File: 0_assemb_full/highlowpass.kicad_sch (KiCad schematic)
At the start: 21 parts, among them U3 LM2902, U4 LM2902

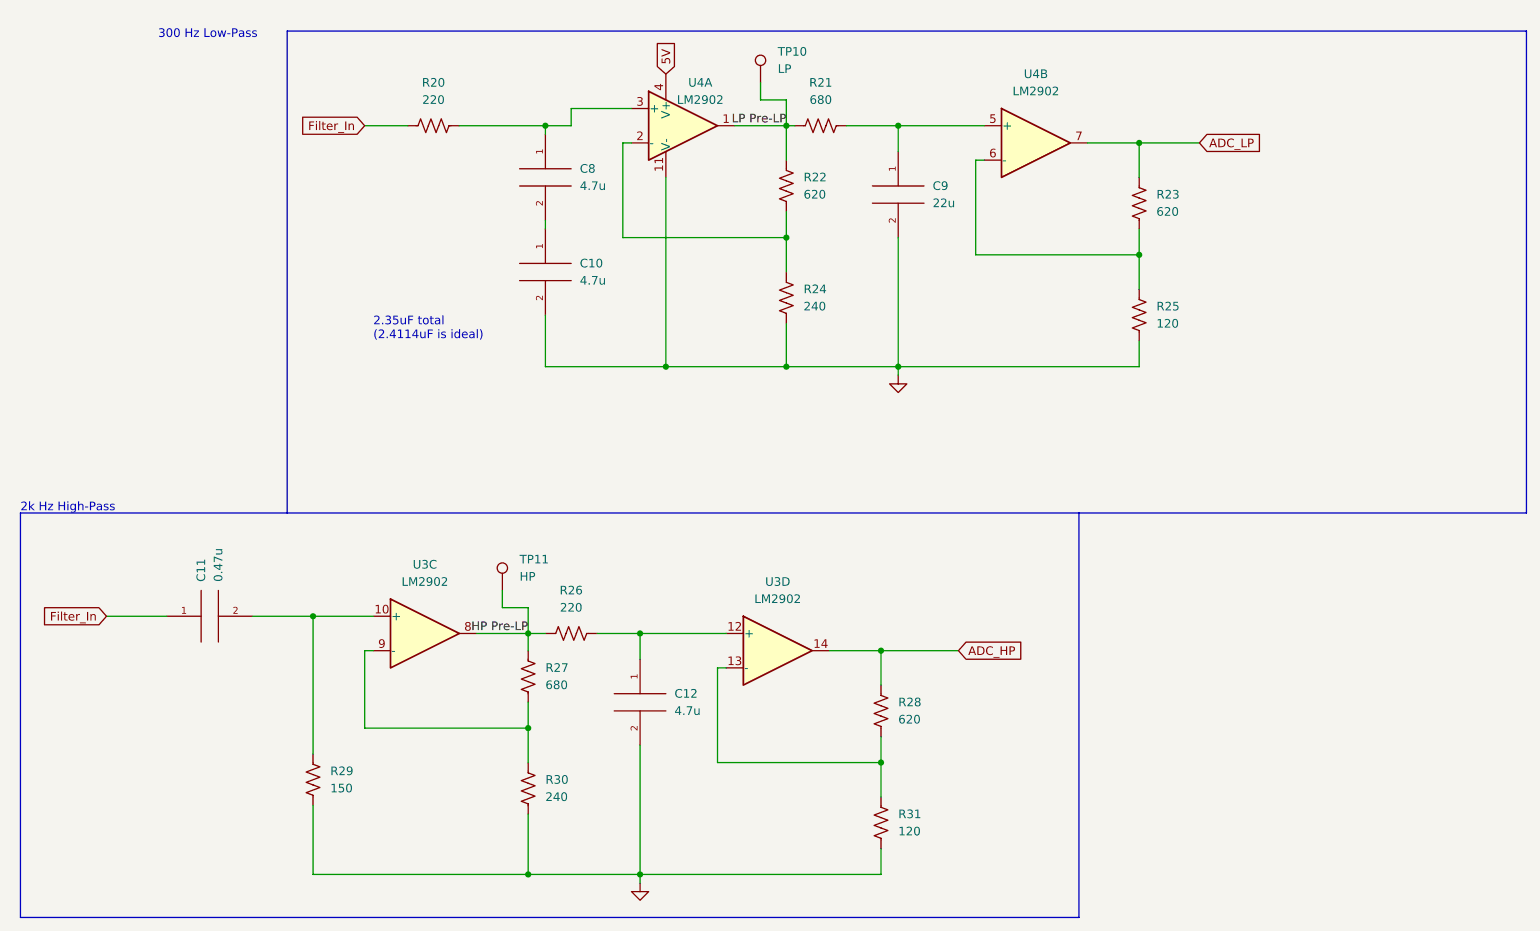
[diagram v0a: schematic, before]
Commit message: Some filter adjustments
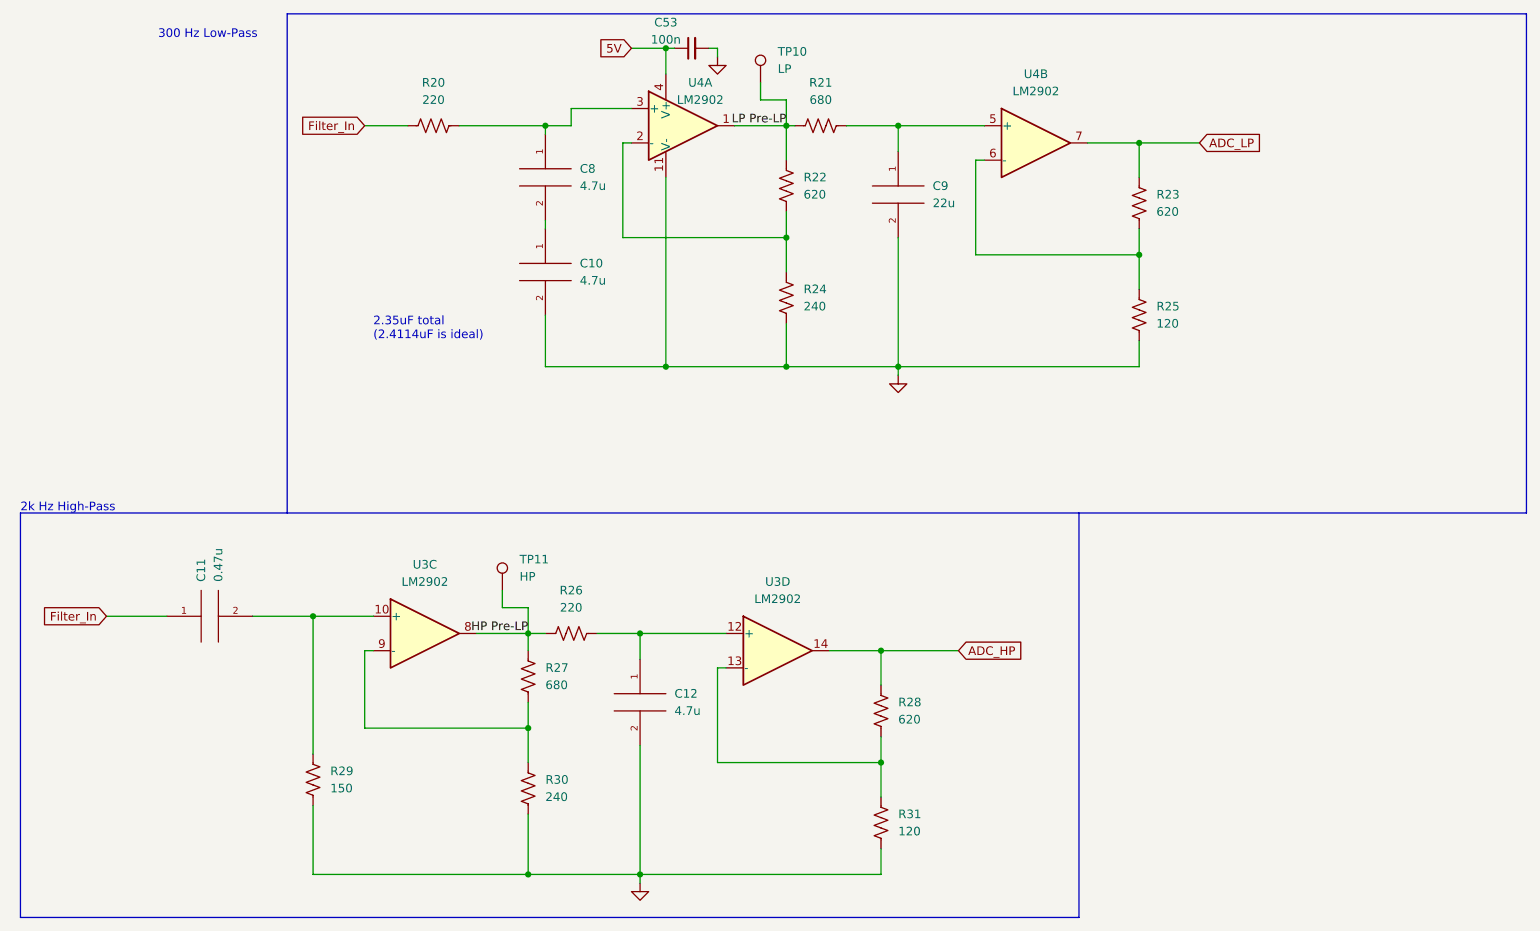
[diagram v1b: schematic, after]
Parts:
- added C53: 100n, Capacitor_SMD:C_0805_2012Metric_Pad1.18x1.45mm_HandSolder, symbol Device:C_Small
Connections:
- net 5V: now also C53.1
- net GND: now also C53.2
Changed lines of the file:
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@@
   (junction (at 179.07 31.75) (diameter 0) (color 0 0 0 0)
   )
+  (junction (at 109.22 17.78) (diameter 0) (color 0 0 0 0)
+  )
   (wire (pts (xy 143.51 45.72) (xy 143.51 64.77))
     (stroke (width 0) (type default) (color 0 0 0 0))
@@
     (stroke (width 0) (type default) (color 0 0 0 0))
   )
-  (polyline (pts (xy 236.22 86.36) (xy 236.22 15.24))
+  (polyline (pts (xy 236.22 86.36) (xy 236.22 12.7))
     (stroke (width 0) (type default) (color 0 0 0 0))
   )
@@
     (stroke (width 0) (type default) (color 0 0 0 0))
   )
-  (polyline (pts (xy 236.22 15.24) (xy 53.34 15.24))
+  (polyline (pts (xy 236.22 12.7) (xy 53.34 12.7))
     (stroke (width 0) (type default) (color 0 0 0 0))
   )
@@
     (stroke (width 0) (type default) (color 0 0 0 0))
   )
+  (wire (pts (xy 109.22 17.78) (xy 110.49 17.78))
+    (stroke (width 0) (type default) (color 0 0 0 0))
+  )
   (wire (pts (xy 127 29.21) (xy 127 34.29))
     (stroke (width 0) (type default) (color 0 0 0 0))
@@
     (stroke (width 0) (type default) (color 0 0 0 0))
   )
+  (wire (pts (xy 116.84 19.05) (xy 116.84 17.78))
+    (stroke (width 0) (type default) (color 0 0 0 0))
+  )
   (wire (pts (xy 88.9 100.33) (xy 88.9 104.14))
     (stroke (width 0) (type default) (color 0 0 0 0))
   )
-  (polyline (pts (xy 53.34 15.24) (xy 53.34 86.36))
+  (polyline (pts (xy 53.34 12.7) (xy 53.34 86.36))
     (stroke (width 0) (type default) (color 0 0 0 0))
   )
@@
     (stroke (width 0) (type default) (color 0 0 0 0))
   )
+  (wire (pts (xy 104.14 17.78) (xy 109.22 17.78))
+    (stroke (width 0) (type default) (color 0 0 0 0))
+  )
   (wire (pts (xy 104.14 31.75) (xy 102.87 31.75))
     (stroke (width 0) (type default) (color 0 0 0 0))
   )
+  (wire (pts (xy 116.84 17.78) (xy 115.57 17.78))
+    (stroke (width 0) (type default) (color 0 0 0 0))
+  )
   (wire (pts (xy 88.9 114.3) (xy 88.9 118.11))
     (stroke (width 0) (type default) (color 0 0 0 0))
@@
   )
   (wire (pts (xy 88.9 118.11) (xy 88.9 123.19))
+    (stroke (width 0) (type default) (color 0 0 0 0))
+  )
+  (wire (pts (xy 109.22 17.78) (xy 109.22 21.59))
     (stroke (width 0) (type default) (color 0 0 0 0))
   )
@@
     (effects (font (size 1.27 1.27)) (justify right bottom))
   )
-  (global_label "5V" (shape input) (at 109.22 21.59 90) (fields_autoplaced)
-    (effects (font (size 1.27 1.27)) (justify left))
-    (property "Intersheet References" "${INTERSHEET_REFS}" (id 0) (at 109.1406 16.8788 90)
-      (effects (font (size 1.27 1.27)) (justify left) hide)
+  (global_label "5V" (shape input) (at 104.14 17.78 180) (fields_autoplaced)
+    (effects (font (size 1.27 1.27)) (justify right))
+    (property "Intersheet References" "${INTERSHEET_REFS}" (id 0) (at 99.4288 17.8594 0)
+      (effects (font (size 1.27 1.27)) (justify right) hide)
     )
   )
@@
     (pin "2")
   )
+  (symbol (lib_id "Device:C_Small") (at 113.03 17.78 90) (unit 1)
+    (in_bom yes) (on_board yes)
+    (property "Reference" "C53" (id 0) (at 109.22 13.97 90))
+    (property "Value" "100n" (id 1) (at 109.22 16.51 90))
+    (property "Footprint" "Capacitor_SMD:C_0805_2012Metric_Pad1.18x1.45mm_HandSolder" (id 2) (at 113.03 17.78 0)
+      (effects (font (size 1.27 1.27)) hide)
+    )
+    (property "Datasheet" "~" (id 3) (at 113.03 17.78 0)
+      (effects (font (size 1.27 1.27)) hide)
+    )
+    (pin "1")
+    (pin "2")
+  )
   (symbol (lib_id "Amplifier_Operational:LM2902") (at 163.83 31.75 0) (unit 2)
     (in_bom yes) (on_board yes) (fields_autoplaced)
@@
     (pin "4")
   )
+  (symbol (lib_id "power:GND") (at 116.84 19.05 0) (unit 1)
+    (in_bom yes) (on_board yes) (fields_autoplaced)
+    (property "Reference" "#PWR048" (id 0) (at 116.84 25.4 0)
+      (effects (font (size 1.27 1.27)) hide)
+    )
+    (property "Value" "GND" (id 1) (at 116.84 24.13 0)
+      (effects (font (size 1.27 1.27)) hide)
+    )
+    (property "Footprint" "" (id 2) (at 116.84 19.05 0)
+      (effects (font (size 1.27 1.27)) hide)
+    )
+    (property "Datasheet" "" (id 3) (at 116.84 19.05 0)
+      (effects (font (size 1.27 1.27)) hide)
+    )
+    (pin "1")
+  )
   (symbol (lib_id "pspice:C") (at 105.41 114.3 0) (unit 1)
